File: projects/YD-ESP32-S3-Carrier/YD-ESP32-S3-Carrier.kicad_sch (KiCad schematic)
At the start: 36 parts, among them J1 YD-ESP32-S3_L, J2 YD-ESP32-S3_R, J3 ES8311_AUDIO, J4 TFT_1.77, J5 BAT_3V7, J6 SPARE_IO_A, J7 SPARE_IO_B, J9 UART1, SW1 VOL_UP, SW2 VOL_DN, SW3 ACTIVATE, SW4 RESET, SW5 POWER_ON_OFF, U1 TP4056, U2 MT3608

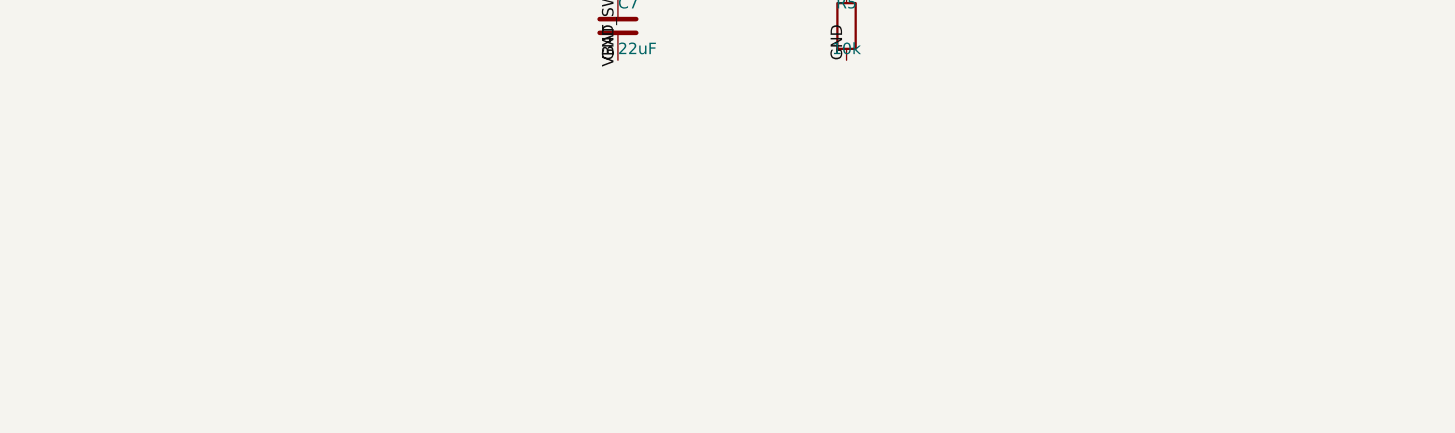
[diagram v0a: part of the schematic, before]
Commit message: 修改位置
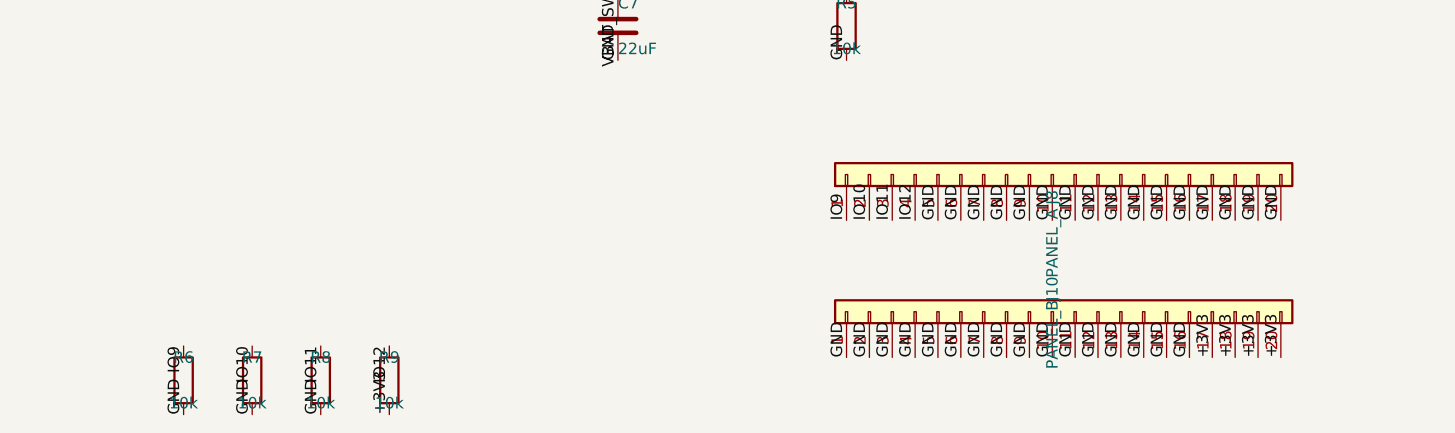
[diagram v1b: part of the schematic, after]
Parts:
- added J10: PANEL_B, Connector_PinHeader_2.54mm:PinHeader_1x20_P2.54mm_Vertical, symbol Connector_Generic:Conn_01x20
- added J8: PANEL_A, Connector_PinHeader_2.54mm:PinHeader_1x20_P2.54mm_Vertical, symbol Connector_Generic:Conn_01x20
- added R6, R7, R8, R9: 10k, Resistor_SMD:R_0603_1608Metric, symbol Device:R
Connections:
- net +3V3: now also J10.17 (Pin_17), J10.18 (Pin_18), J10.19 (Pin_19), J10.20 (Pin_20), R9.2
- net GND: now also J10.1 (Pin_1), J10.10 (Pin_10), J10.11 (Pin_11), J10.12 (Pin_12), J10.13 (Pin_13), J10.14 (Pin_14), J10.15 (Pin_15), J10.16 (Pin_16), J10.2 (Pin_2), J10.3 (Pin_3), J10.4 (Pin_4), J10.5 (Pin_5), J10.6 (Pin_6), J10.7 (Pin_7), J10.8 (Pin_8), J10.9 (Pin_9), J8.10 (Pin_10), J8.11 (Pin_11), J8.12 (Pin_12), J8.13 (Pin_13), J8.14 (Pin_14), J8.15 (Pin_15), J8.16 (Pin_16), J8.17 (Pin_17), J8.18 (Pin_18), J8.19 (Pin_19), J8.20 (Pin_20), J8.5 (Pin_5), J8.6 (Pin_6), J8.7 (Pin_7), J8.8 (Pin_8), J8.9 (Pin_9), R6.2, R7.2, R8.2
- net IO10: now also J8.2 (Pin_2), R7.1
- net IO11: now also J8.3 (Pin_3), R8.1
- net IO12: now also J8.4 (Pin_4), R9.1
- net IO9: now also J8.1 (Pin_1), R6.1
